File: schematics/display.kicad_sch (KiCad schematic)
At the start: 64 parts, among them Q1 S9012, Q10 2N3904, Q11 2N3904, Q12 2N3904, Q13 2N3904, Q14 2N3904, Q15 2N3904, Q16 2N3904, Q17 2N3904, Q2 S9012, Q3 S9012, Q4 S9012, Q5 S9012, Q6 S9012, Q7 S9012, Q8 S9012, Q9 2N3904, U12 74HC138, U13 5161BS, U14 74HC251, U15 5161BS, U16 74HC251, U17 5161BS, U18 5161BS, U19 74HC251, U20 5161BS, U21 5161BS, U22 74HC251, U23 74HC4511, U24 5161BS, U25 5161BS, U26 5161BS

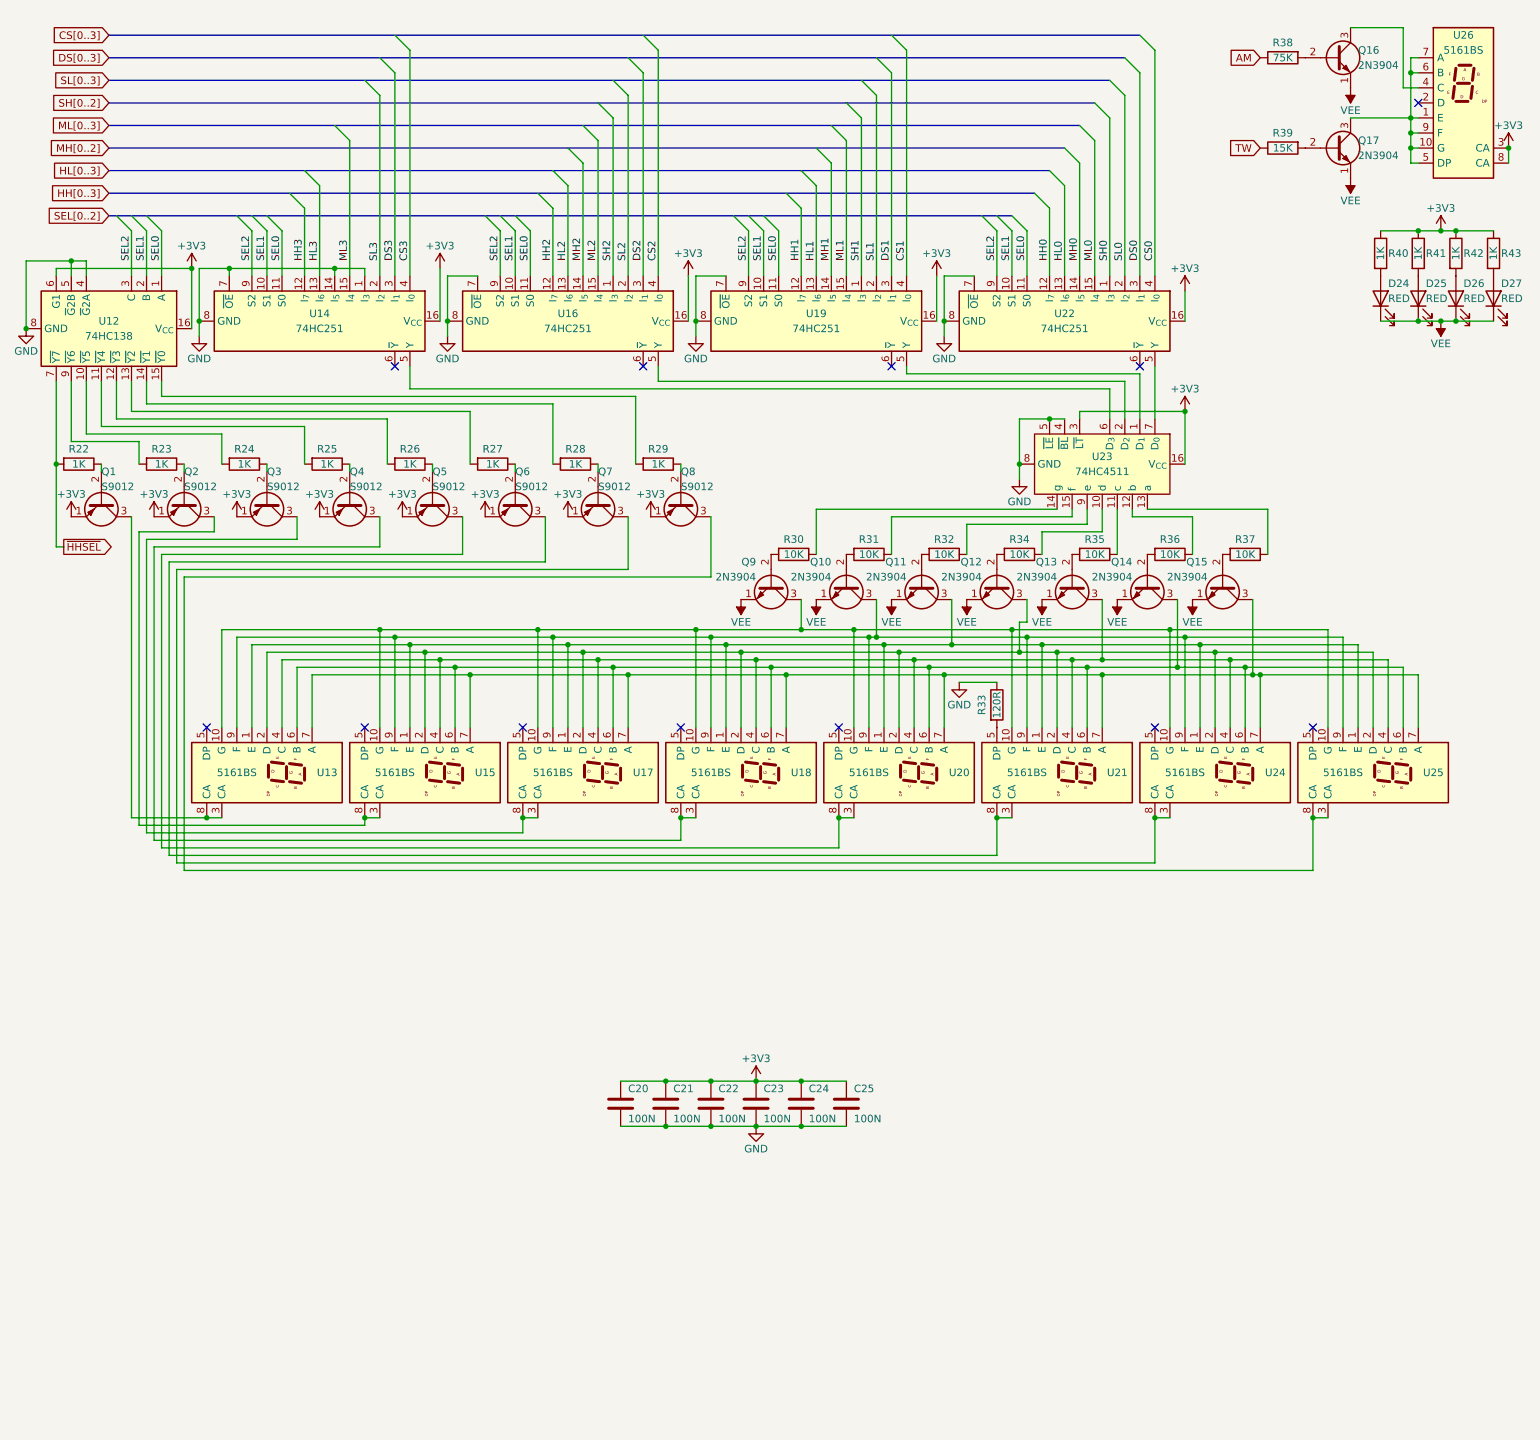
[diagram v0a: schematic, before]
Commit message: 24-12 converter cleanup
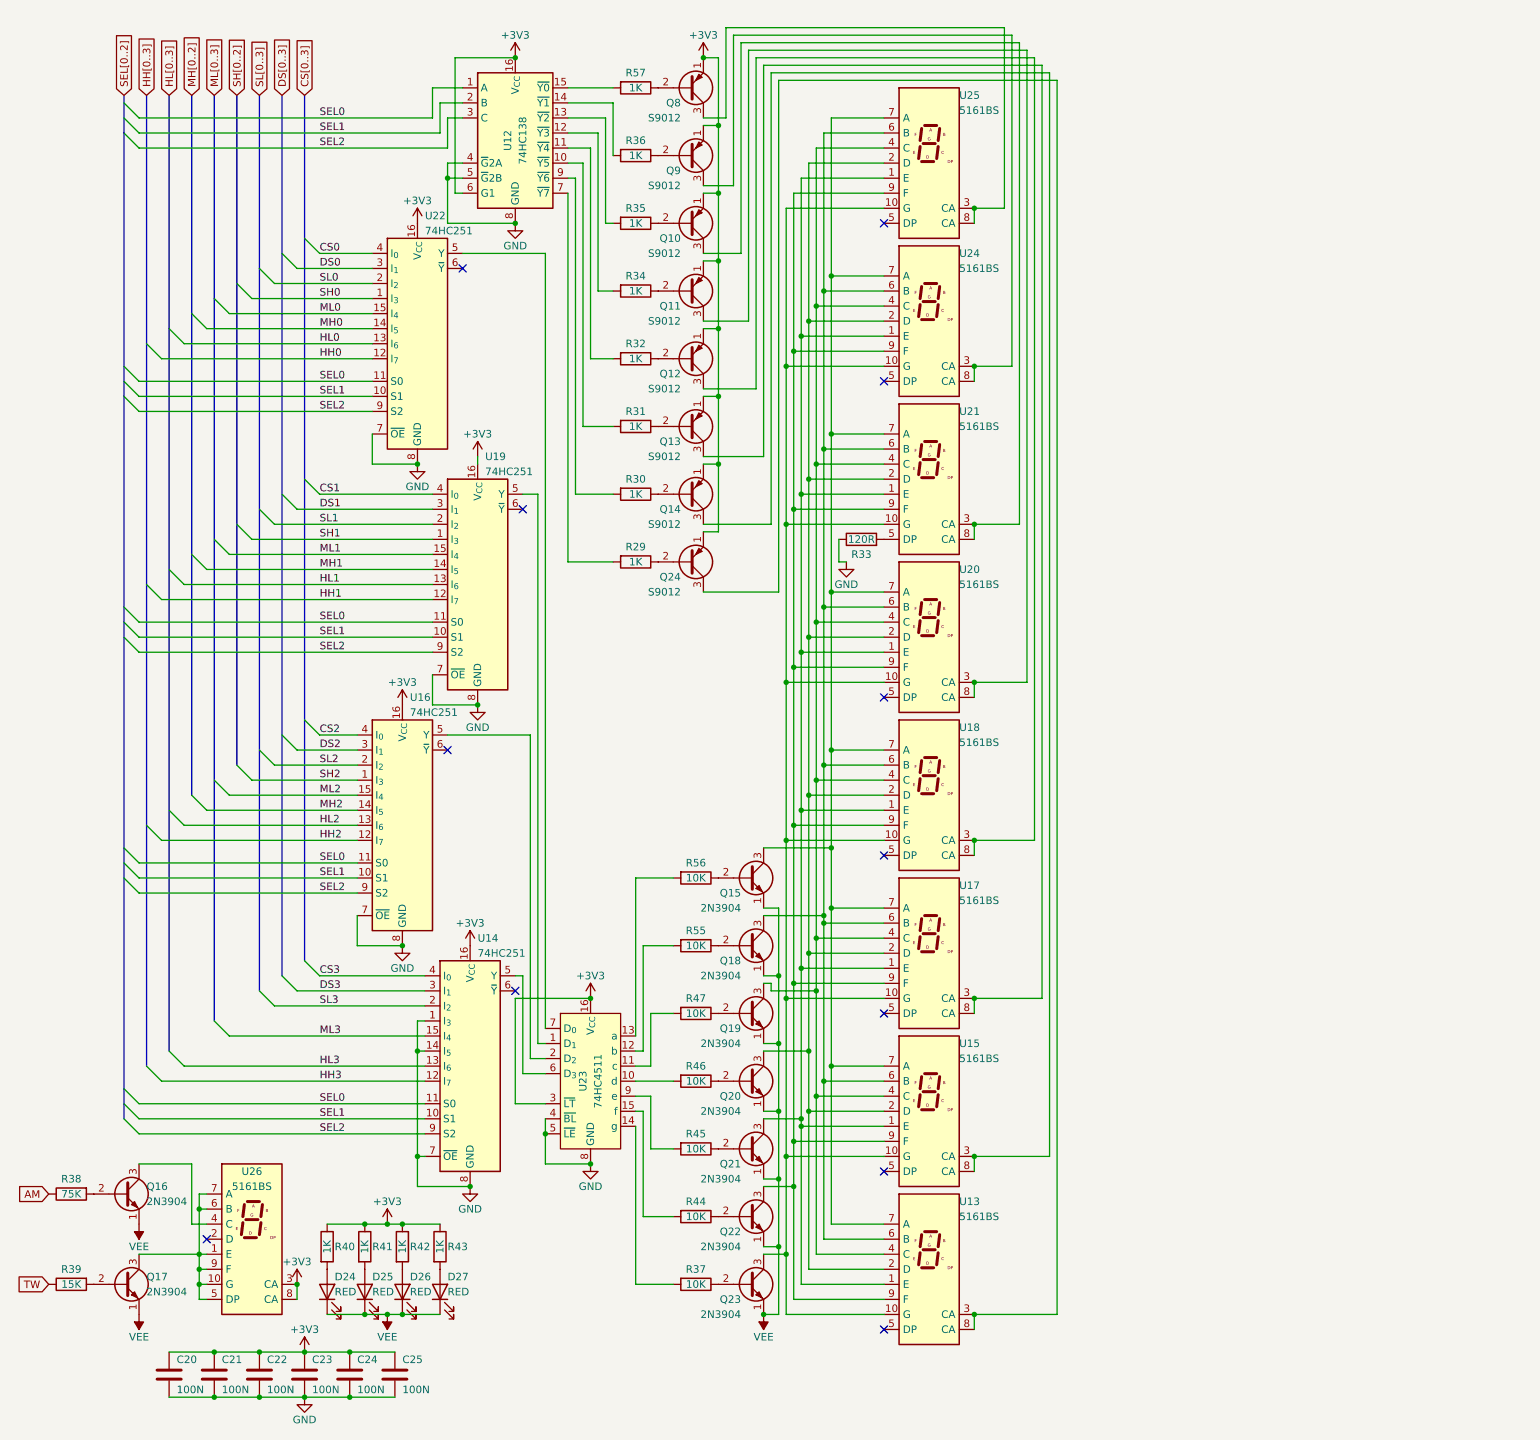
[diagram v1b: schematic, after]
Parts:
- removed Q1, Q2, Q3, Q4, Q5, Q6, Q7: S9012, Package_TO_SOT_THT:TO-92_Inline, symbol Transistor_BJT:Q_PNP_EBC
- removed Q10, Q11, Q12, Q13, Q14, Q9: 2N3904, Package_TO_SOT_THT:TO-92_Inline, symbol Transistor_BJT:2N3904
- removed R22, R23, R24, R25, R26, R27, R28: 1K, symbol Device:R
- added Q10, Q11, Q12, Q13, Q14, Q24, Q9: S9012, Package_TO_SOT_THT:TO-92_Inline, symbol Transistor_BJT:Q_PNP_EBC
- added Q18, Q19, Q20, Q21, Q22, Q23: 2N3904, Package_TO_SOT_THT:TO-92_Inline, symbol Transistor_BJT:2N3904
- added R44, R45, R46, R47, R55, R56: 10K, symbol Device:R
- added R57: 1K, symbol Device:R
- R30, R31, R32, R34, R35, R36: value 10K -> 1K
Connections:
- net +3V3: now also Q10.1 (E), Q11.1 (E), Q12.1 (E), Q13.1 (E), Q14.1 (E), Q24.1 (E), Q9.1 (E)
- net VEE: now also Q18.1 (E), Q19.1 (E), Q20.1 (E), Q21.1 (E), Q22.1 (E), Q23.1 (E)
- net at R36.2: now also U12.14 (~{Y1})
- net at U13.6 (B), U15.6 (B), U17.6 (B)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: now also Q18.3 (C)
- net at U13.1 (E), U15.1 (E), U17.1 (E)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: now also Q21.3 (C)
- net at U13.10 (G), U15.10 (G), U17.10 (G)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: now also Q23.3 (C)
- net at U13.2 (D), U15.2 (D), U17.2 (D)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: now also Q20.3 (C)
- net at U21.3 (CA), U21.8 (CA): now also Q10.3 (C)
- net at U13.4 (C), U15.4 (C), U17.4 (C)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: now also Q19.3 (C)
- net at U13.9 (F), U15.9 (F), U17.9 (F)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: now also Q22.3 (C)
- net at R34.2: now also U12.12 (~{Y3})
- net at R32.1: now also Q12.2 (B); no longer U23.9 (e)
- net at R32.2: now also U12.11 (~{Y4})
- net at R37.2: now also U23.14 (g); no longer Q15.2 (B)
- net at R30.2: now also U12.9 (~{Y6})
- net at R29.1: now also Q24.2 (B); no longer Q8.2 (B)
- net at U18.3 (CA), U18.8 (CA): now also Q12.3 (C)
- net at U12.15 (~{Y0}): now also R57.2; no longer R29.2
- net at U20.3 (CA), U20.8 (CA): now also Q11.3 (C)
- net at R31.1: now also Q13.2 (B); no longer U23.15 (f)
- net at R31.2: now also U12.10 (~{Y5})
- net at U17.3 (CA), U17.8 (CA): now also Q13.3 (C)
- net at U12.13 (~{Y2}): now also R35.2
- net at U23.10 (d): now also R46.2; no longer R34.1
- net at U23.11 (c): now also R47.2; no longer R35.1
- net at U23.12 (b): now also R55.2; no longer R36.1
- net at R37.1: now also Q23.2 (B); no longer U23.13 (a)
- net at R30.1: now also Q14.2 (B); no longer U23.14 (g)
- net at U24.3 (CA), U24.8 (CA): now also Q9.3 (C)
- net at U15.3 (CA), U15.8 (CA): now also Q14.3 (C)
- net at U13.3 (CA), U13.8 (CA): now also Q24.3 (C)
- net ~{HHSEL}: no longer names the net of U12.7 (~{Y7})
- net ~{HHSEL}: now also R29.2
- new net: Q19.2 (B), R47.1
- new net: Q18.2 (B), R55.1
- new net: Q10.2 (B), R35.1
- new net: Q8.2 (B), R57.1
- new net: Q20.2 (B), R46.1
- new net: Q22.2 (B), R44.1
- new net: R44.2, U23.15 (f)
- new net: Q21.2 (B), R45.1
- new net: Q11.2 (B), R34.1
- new net: Q15.2 (B), R56.1
- new net: R56.2, U23.13 (a)
- new net: Q9.2 (B), R36.1
- new net: R45.2, U23.9 (e)
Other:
- moved on the sheet: C20, C21, C22, C23, C24, C25, D24, D25, D26, D27, Q16, Q17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
